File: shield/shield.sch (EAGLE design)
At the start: 10 parts, among them IC1 74HC594N, IC2 74HC594N

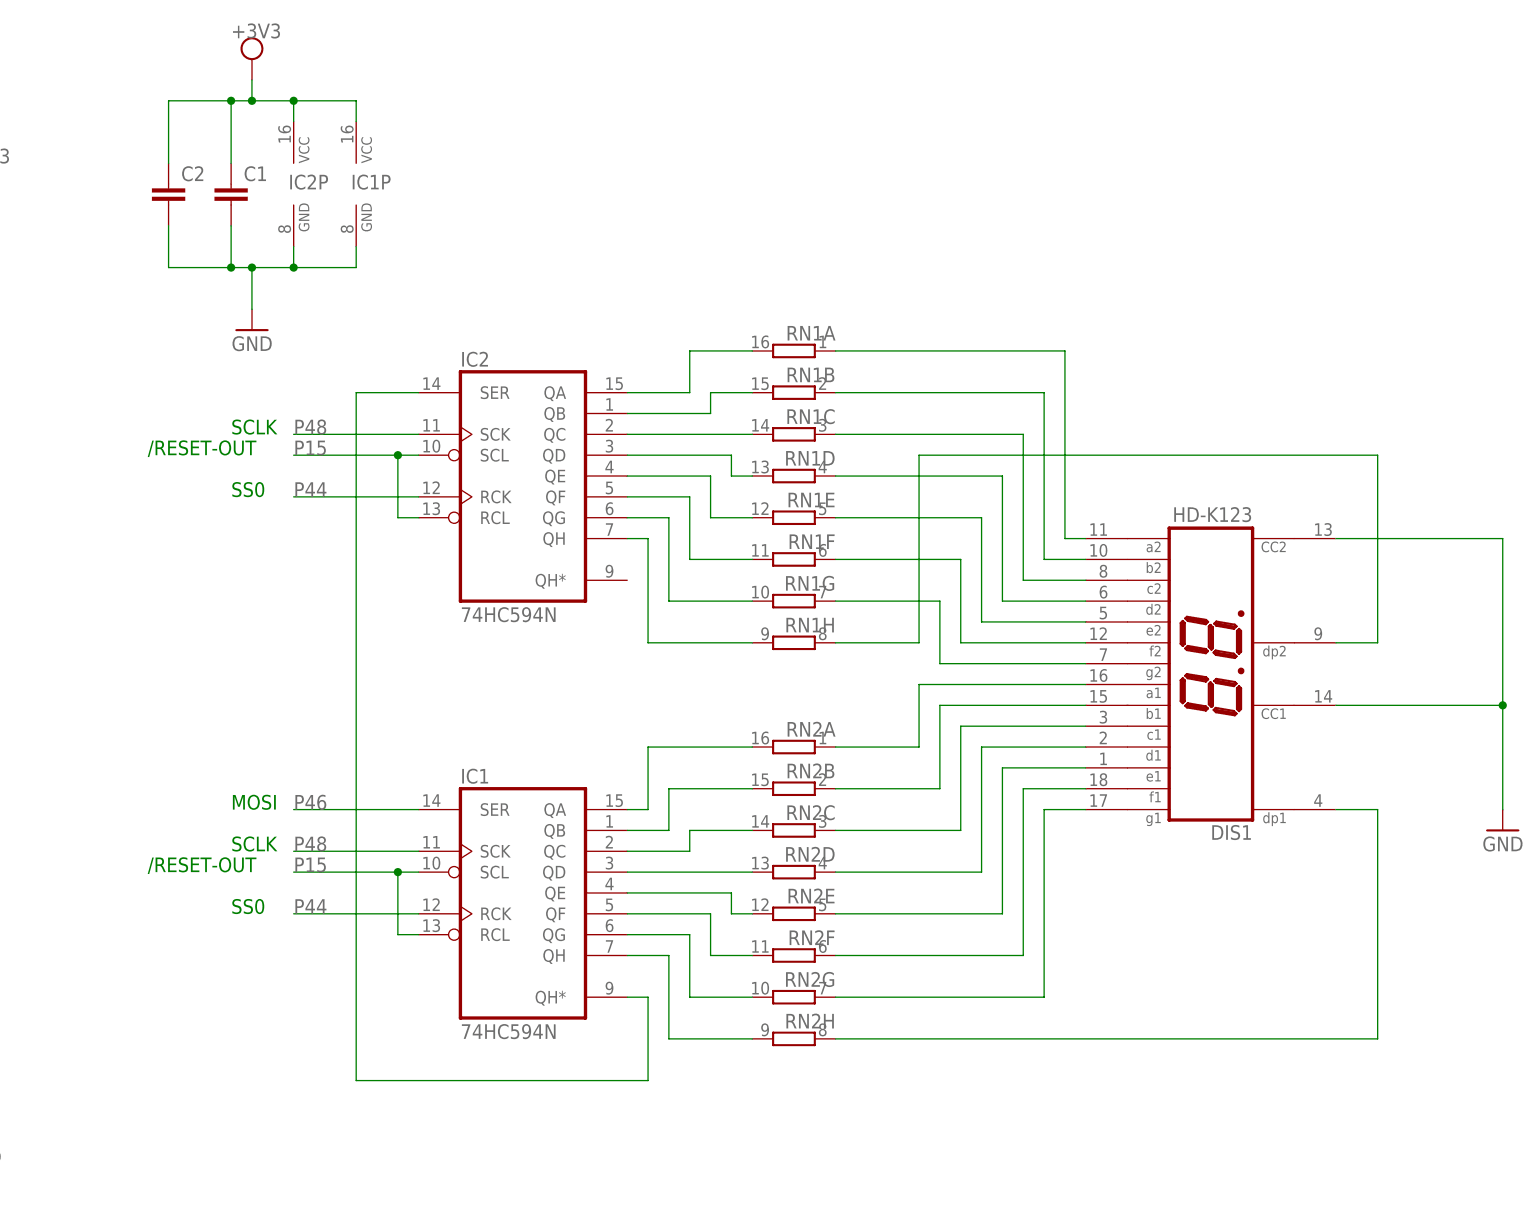
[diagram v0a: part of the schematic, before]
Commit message: Update schematic
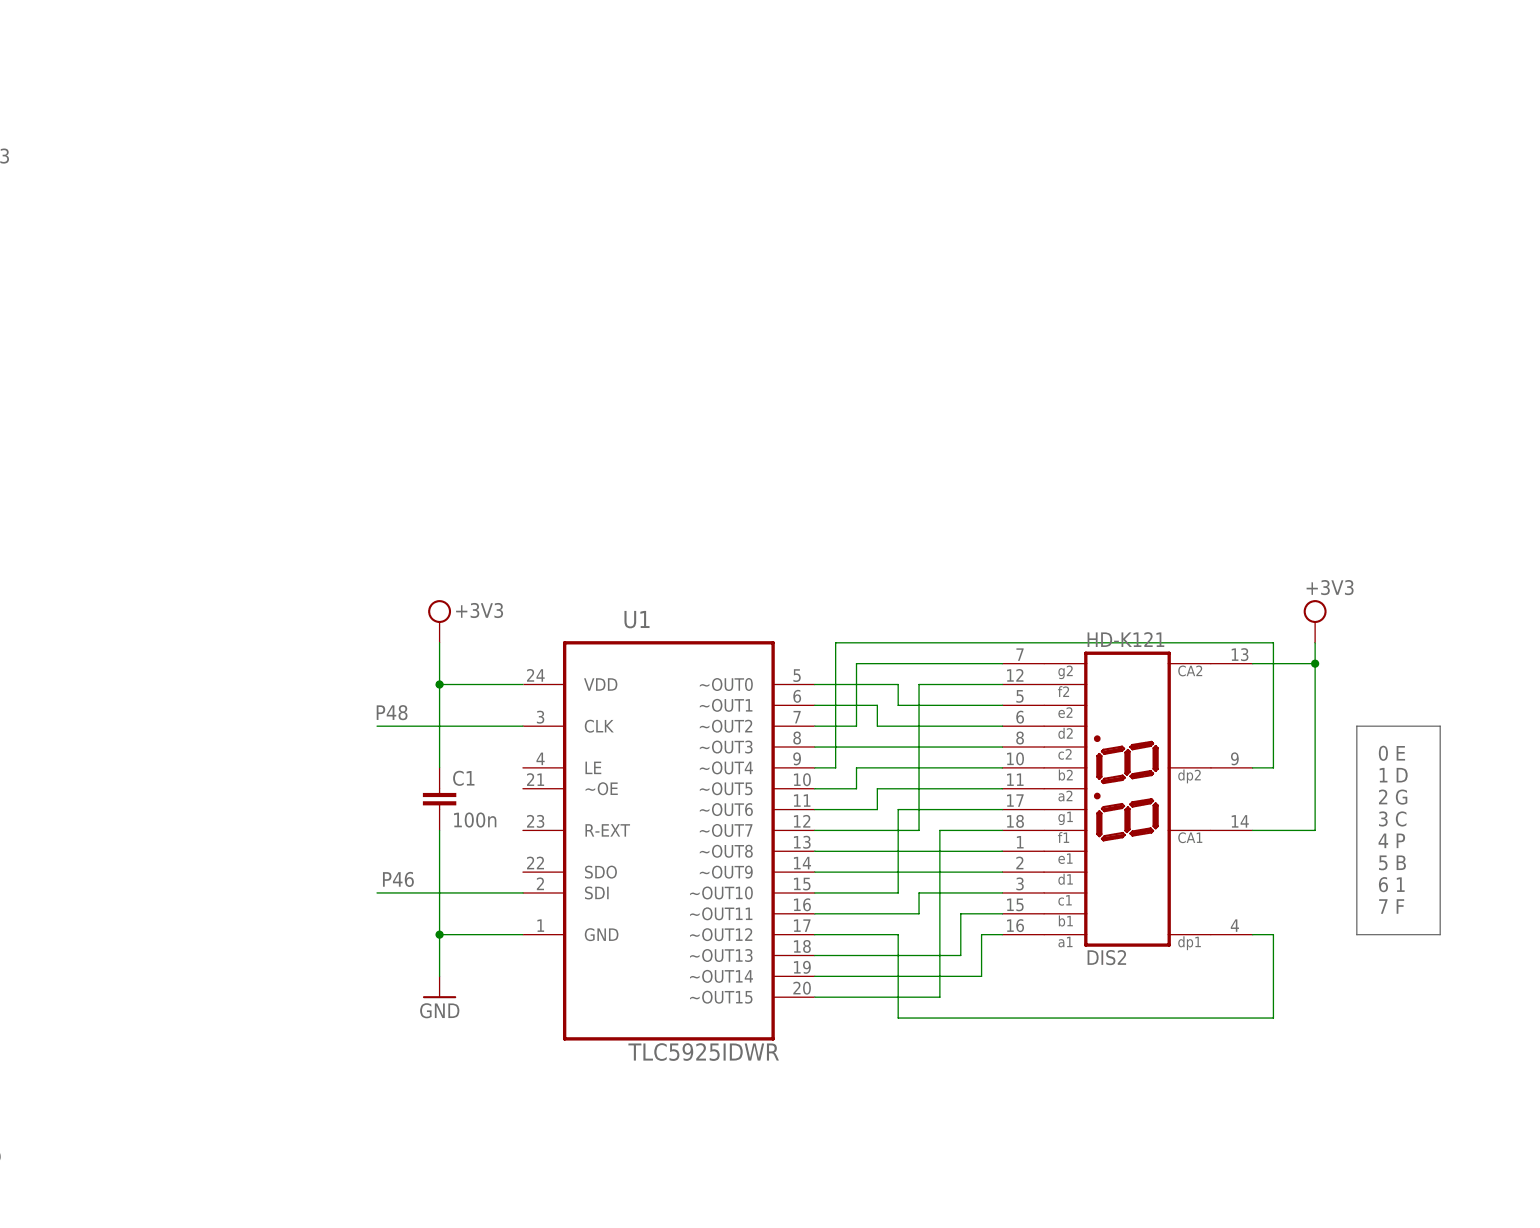
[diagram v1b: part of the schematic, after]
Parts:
- removed C2: (no value), rcl:C-EU025-030X050
- removed DIS1: HD-K123, display-hp:HD-K123
- removed IC1, IC2: 74HC594N, 74xx-eu:74HC594N
- removed RN1, RN2: (no value), resistor-dil:8R-N
- added DIS2: HD-K121, display-hp:HD-K121
- added U1: TLC5925IDWR, Texas Instruments_By_element14_Batch_1:TLC5925IDWR
- C1: value (none) -> 100n; device rcl:C-EU025-030X050 -> capacitor-wima:C2.5/2
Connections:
- removed net N$17: IC1A.QH*, IC2A.SER
- removed net N$18: DIS1.A2, RN1A.1
- removed net N$19: DIS1.B2, RN1B.1
- removed net N$20: DIS1.C2, RN1C.1
- removed net N$21: DIS1.D2, RN1D.1
- removed net N$22: DIS1.E2, RN1E.1
- removed net N$23: DIS1.F2, RN1F.1
- removed net N$24: DIS1.G2, RN1G.1
- removed net N$25: DIS1.G1, RN2G.1
- removed net N$26: DIS1.A1, RN2A.1
- removed net N$27: DIS1.B1, RN2B.1
- removed net N$28: DIS1.C1, RN2C.1
- removed net N$29: DIS1.D1, RN2D.1
- removed net N$30: DIS1.E1, RN2E.1
- removed net N$31: DIS1.F1, RN2F.1
- removed net N$32: DIS1.DP2, RN1H.1
- removed net N$33: DIS1.DP1, RN2H.1
- net +3V3: now also DIS2.CA1, DIS2.CA2, U1.VDD; no longer C2.1, IC1P.VCC, IC2P.VCC
- net GND: now also U1.GND; no longer C2.2, DIS1.CC1, DIS1.CC2, IC1P.GND, IC2P.GND
- net N$1: now also DIS2.E2, U1.~OUT0; no longer IC2A.QA, RN1A.2
- net N$10: now also DIS2.D1, U1.~OUT9; no longer IC1A.QB, RN2B.2
- net N$11: now also DIS2.G1, U1.~OUT10; no longer IC1A.QC, RN2C.2
- net N$12: now also DIS2.C1, U1.~OUT11; no longer IC1A.QD, RN2D.2
- net N$13: now also DIS2.DP1, U1.~OUT12; no longer IC1A.QE, RN2E.2
- net N$14: now also DIS2.B1, U1.~OUT13; no longer IC1A.QF, RN2F.2
- net N$15: now also DIS2.A1, U1.~OUT14; no longer IC1A.QG, RN2G.2
- net N$16: now also DIS2.F1, U1.~OUT15; no longer IC1A.QH, RN2H.2
- net N$2: now also DIS2.D2, U1.~OUT1; no longer IC2A.QB, RN1B.2
- net N$3: now also DIS2.G2, U1.~OUT2; no longer IC2A.QC, RN1C.2
- net N$4: now also DIS2.C2, U1.~OUT3; no longer IC2A.QD, RN1D.2
- net N$5: now also DIS2.DP2, U1.~OUT4; no longer IC2A.QE, RN1E.2
- net N$6: now also DIS2.B2, U1.~OUT5; no longer IC2A.QF, RN1F.2
- net N$7: now also DIS2.A2, U1.~OUT6; no longer IC2A.QG, RN1G.2
- net N$8: now also DIS2.F2, U1.~OUT7; no longer IC2A.QH, RN1H.2
- net N$9: now also DIS2.E1, U1.~OUT8; no longer IC1A.QA, RN2A.2
- net P15: no longer IC1A.RCL, IC1A.SCL, IC2A.RCL, IC2A.SCL
- net P44: no longer IC1A.RCK, IC2A.RCK
- net P46: now also U1.SDI; no longer IC1A.SER
- net P48: now also U1.CLK; no longer IC1A.SCK, IC2A.SCK
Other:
- note added: "0 E 1 D 2 G 3 C 4 P 5 B 6 1 7 F"
- note removed: "/RESET-OUT"
- note removed: "MOSI"
- note removed: "SCLK"
- note removed: "SS0"
- moved on the sheet: C1

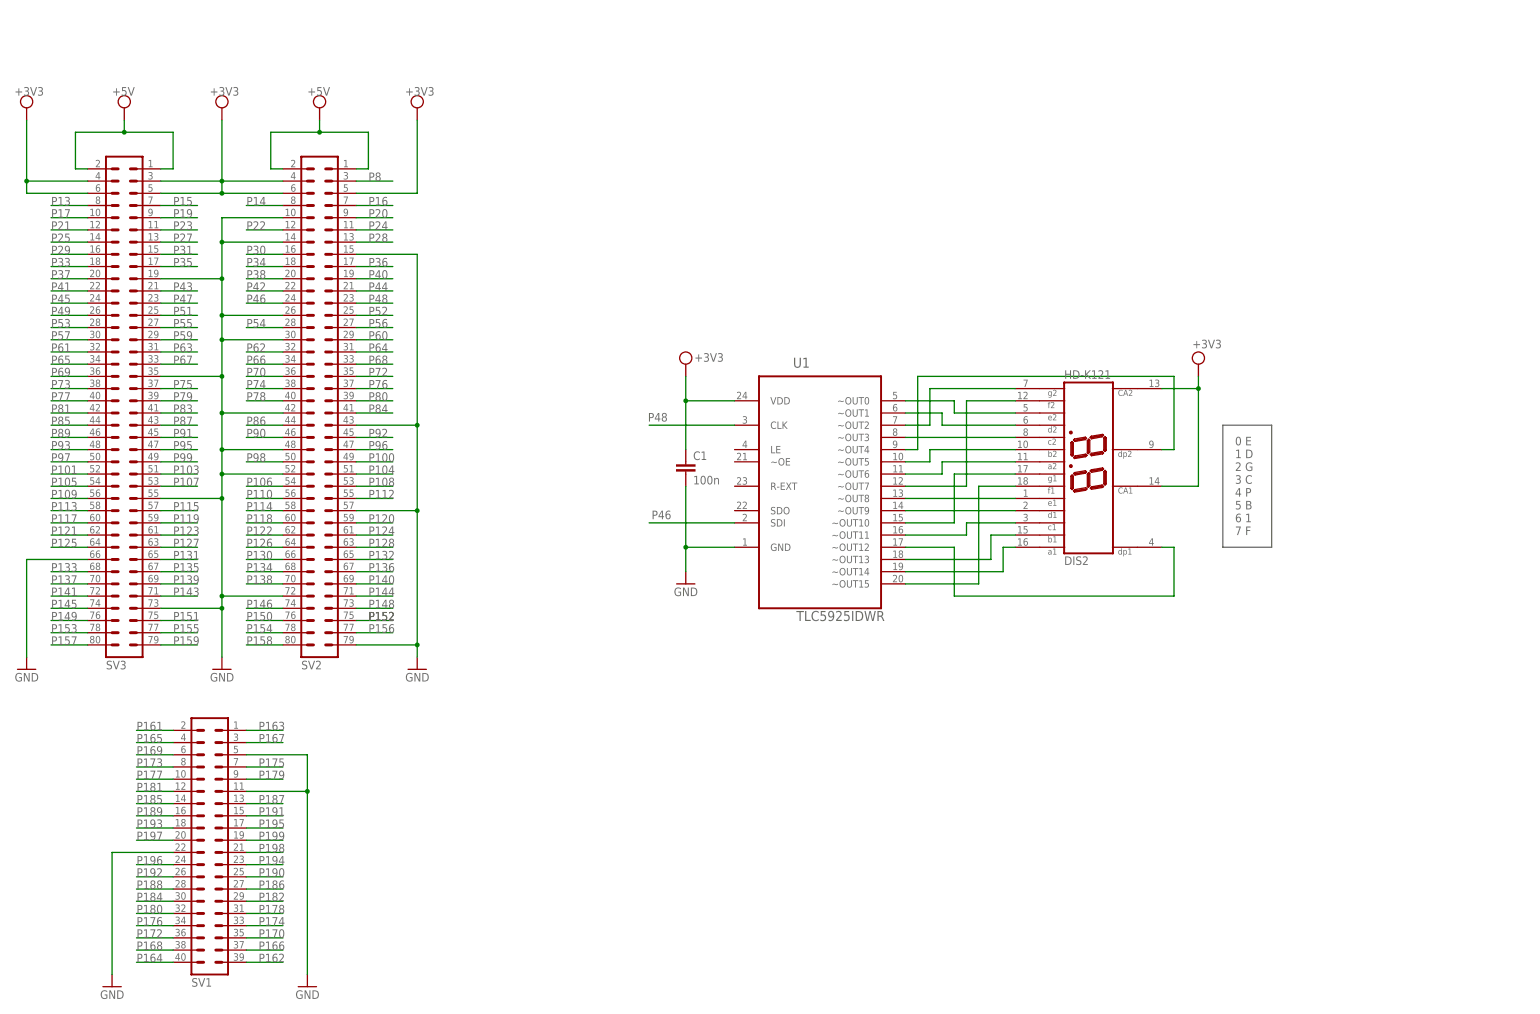
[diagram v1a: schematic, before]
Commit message: Update schematics
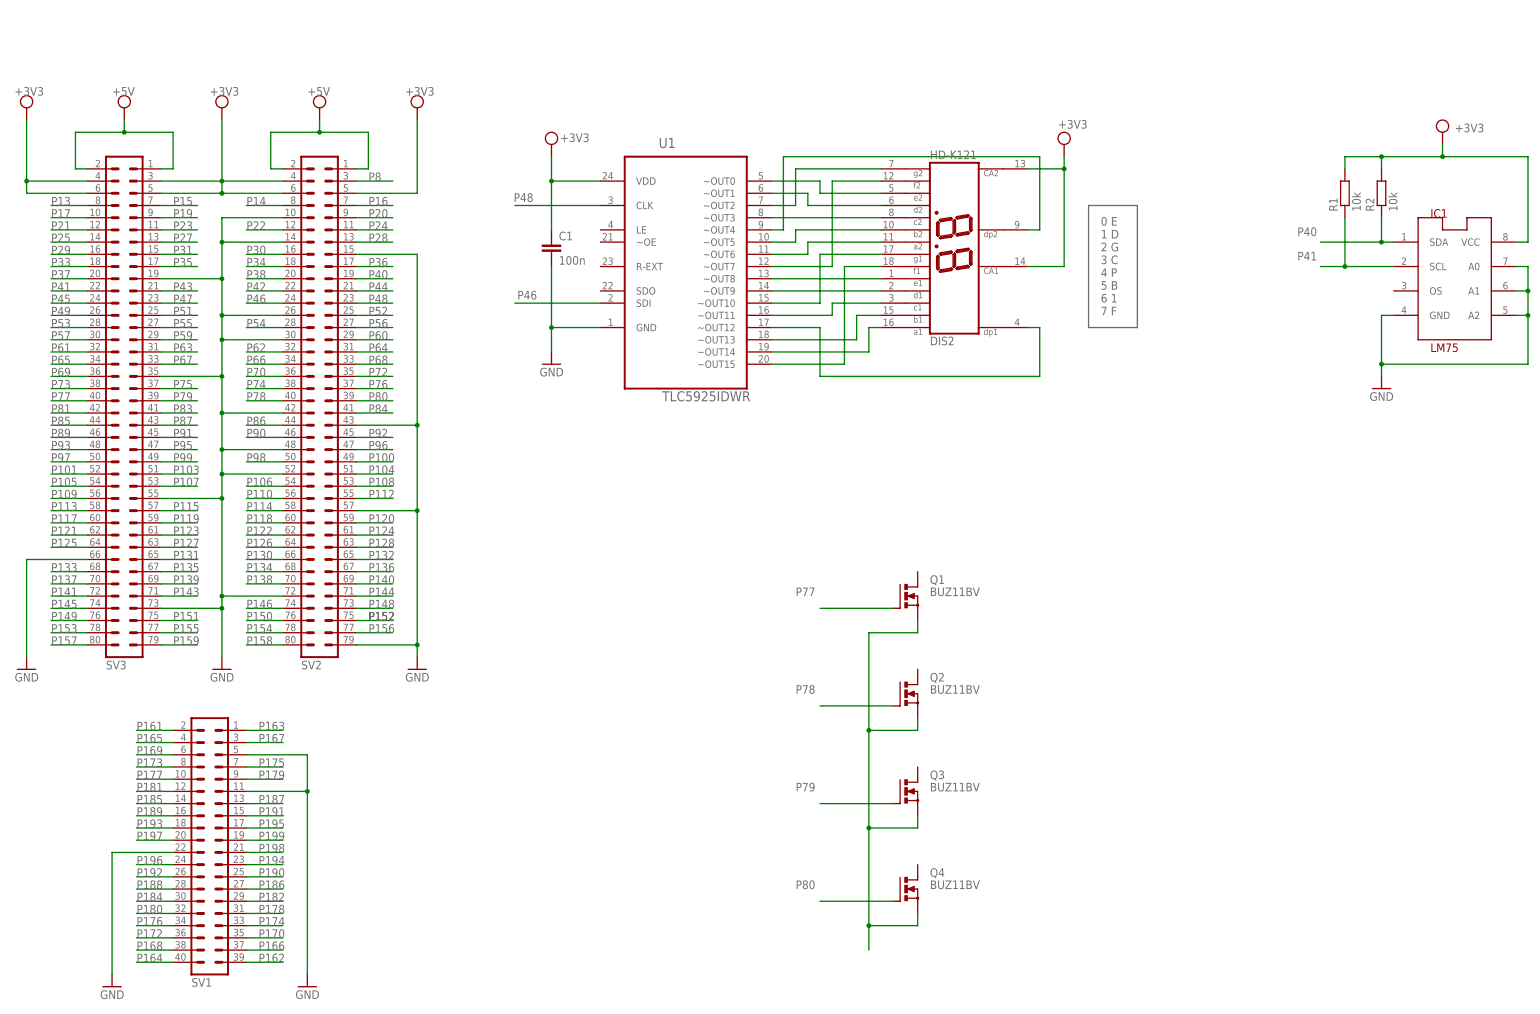
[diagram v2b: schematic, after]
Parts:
- added IC1: LM75, lm75:LM75_ICN
- added Q1, Q2, Q3, Q4: BUZ11BV, transistor-power:BUZ11BV
- added R1, R2: 10k, rcl:R-EU_0207/10
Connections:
- new net N$17: Q1.S, Q2.S, Q3.S, Q4.S
- net +3V3: now also IC1.VCC, R1.2, R2.2
- net GND: now also IC1.A0, IC1.A1, IC1.A2, IC1.GND
- net P40: now also IC1.SDA, R2.1
- net P41: now also IC1.SCL, R1.1
- net P77: now also Q1.G
- net P78: now also Q2.G
- net P79: now also Q3.G
- net P80: now also Q4.G
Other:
- moved on the sheet: C1, DIS2, U1
